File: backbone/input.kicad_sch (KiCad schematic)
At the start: 0 parts

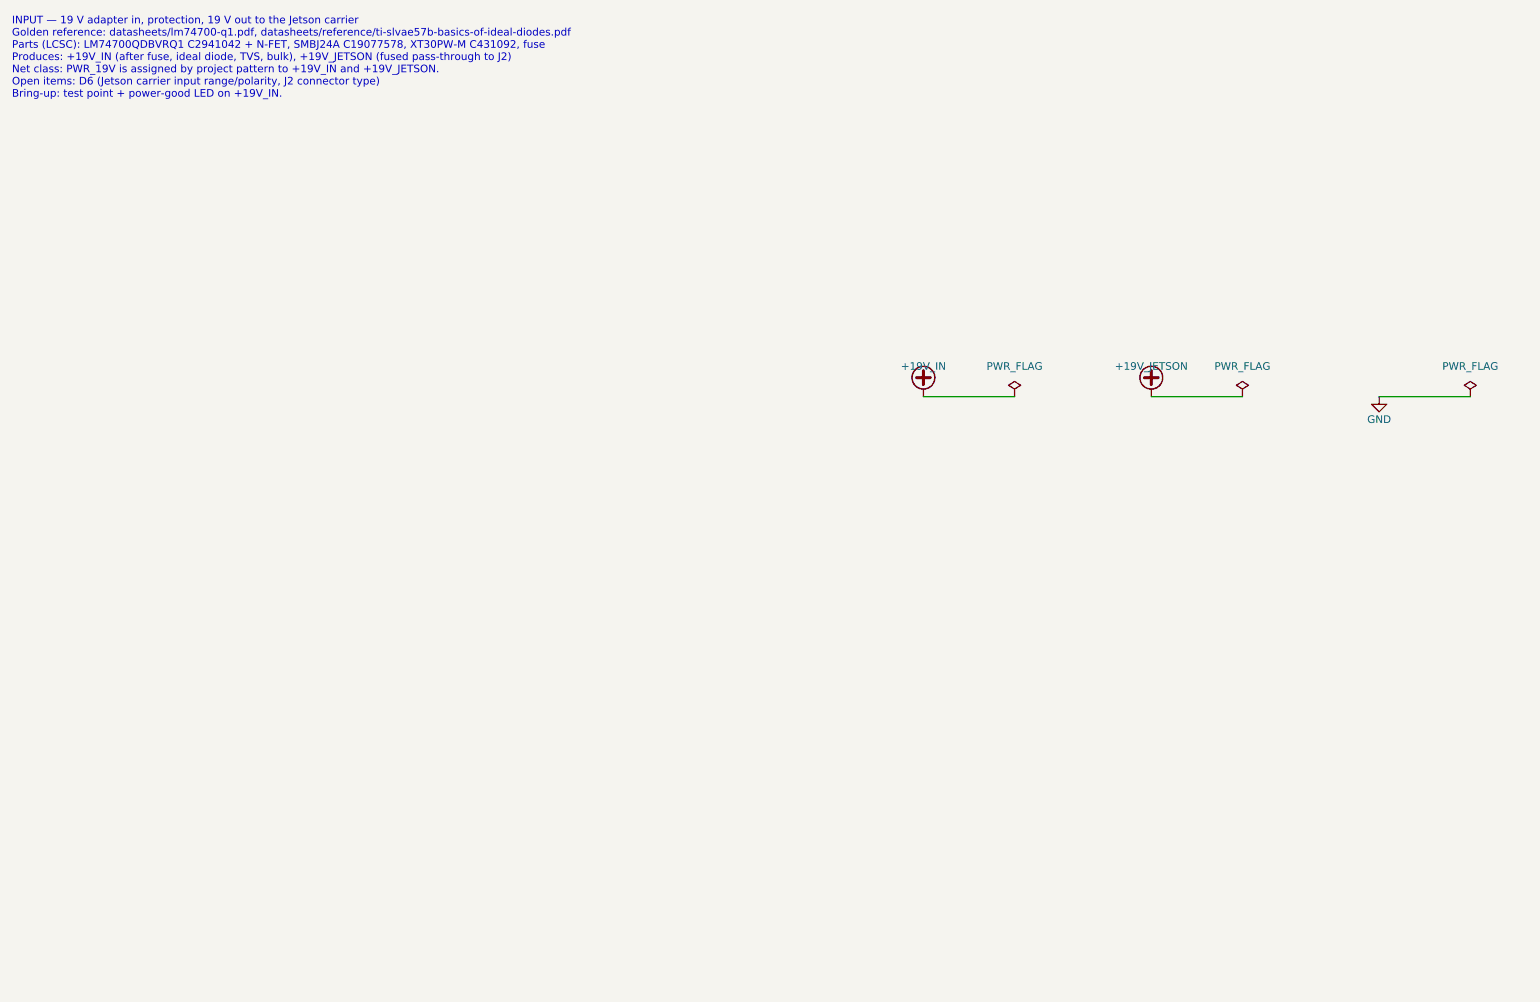
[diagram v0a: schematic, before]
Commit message: before hand editing
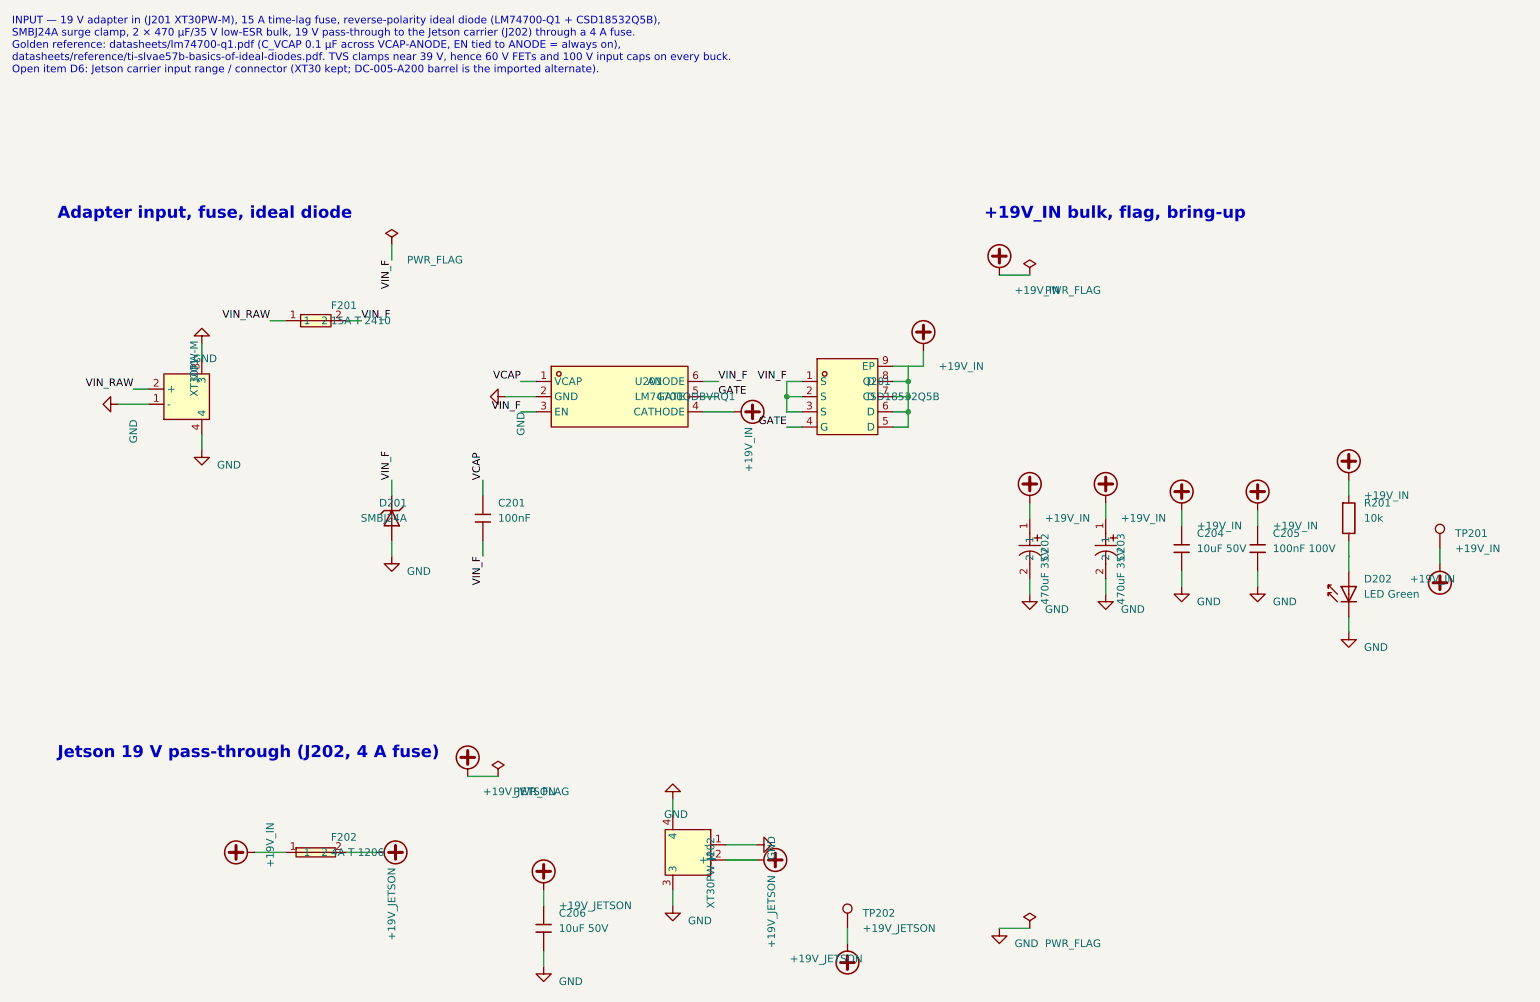
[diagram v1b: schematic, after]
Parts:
- added C201: 100nF, 0_backbone:C_0603, symbol 0_backbone:C_0603
- added C202, C203: 470uF 35V, 0_backbone:CAP-SMD_BD10.0-L10.3-W10.3-LS11.3-FD, symbol 0_backbone:RVE470UF35V167RV084
- added C204, C206: 10uF 50V, 0_backbone:C_1206, symbol 0_backbone:C_1206
- added C205: 100nF 100V, 0_backbone:C_0805, symbol 0_backbone:C_0805
- added D201: SMBJ24A, 0_backbone:D_SMB, symbol 0_backbone:TVS_SMB
- added D202: LED Green, 0_backbone:D_0805, symbol 0_backbone:LED_0805_Green
- added F201: 15A T 2410, 0_backbone:FUSE-SMD_L6.1-W2.7, symbol 0_backbone:0453015.MR
- added F202: 4A T 1206, 0_backbone:F1206, symbol 0_backbone:1206TD-4A
- added J201, J202: XT30PW-M, 0_backbone:CONN-TH_XT30PW-M, symbol 0_backbone:XT30PW-M
- added Q201: CSD18532Q5B, 0_backbone:SON-8_L5.0-W6.0-P1.27-BL-1, symbol 0_backbone:CSD18532Q5B
- added R201: 10k, 0_backbone:R_0603, symbol 0_backbone:R_0603
- added TP201: +19V_IN, 0_backbone:TestPoint_Pad_D1.5mm, symbol 0_backbone:TestPoint
- added TP202: +19V_JETSON, 0_backbone:TestPoint_Pad_D1.5mm, symbol 0_backbone:TestPoint
- added U201: LM74700QDBVRQ1, 0_backbone:SOT-23-6_L2.9-W1.6-P0.95-LS2.8-BL, symbol 0_backbone:LM74700QDBVRQ1
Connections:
- net +19V_IN: now also C202.1, C203.1, C204.1, C205.1, F202.1, Q201.5 (D), Q201.6 (D), Q201.7 (D), Q201.8 (D), Q201.9 (EP), R201.1, TP201.1, U201.4 (CATHODE)
- net +19V_JETSON: now also C206.1, F202.2, J202.2 (+), TP202.1
- net GND: now also C202.2, C203.2, C204.2, C205.2, C206.2, D201.2, D202.1, J201.1 (-), J201.3, J201.4, J202.1 (-), J202.3, J202.4, U201.2 (GND)
- new net: D202.2, R201.2
- new net GATE: Q201.4 (G), U201.5 (GATE)
- new net VCAP: C201.1, U201.1 (VCAP)
- new net VIN_F: C201.2, D201.1, F201.2, Q201.1 (S), Q201.2 (S), Q201.3 (S), U201.3 (EN), U201.6 (ANODE)
- new net VIN_RAW: F201.1, J201.2 (+)
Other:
- note added: "+19V_IN bulk, flag, bring-up"
- note added: "Adapter input, fuse, ideal diode"
- note added: "INPUT — 19 V adapter in (J201 XT30PW-M), 15 A time-lag fuse, reverse-polarity ideal diode (LM74700-Q1 + CSD18532Q5B), SMBJ24A surge clamp, 2 × 470 µF/35 V low-ESR bulk, 19 V pass-through to the Jetson carrier (J202) through a 4 A fuse. Golden reference: datasheets/lm74700-q1.pdf (C_VCAP 0.1 µF across VCAP-ANODE, EN tied to ANODE = always on), datasheets/reference/ti-slvae57b-basics-of-ideal-diode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"
- note added: "Jetson 19 V pass-through (J202, 4 A fuse)"
- note removed: "INPUT — 19 V adapter in, protection, 19 V out to the Jetson carrier Golden reference: datasheets/lm74700-q1.pdf, datasheets/reference/ti-slvae57b-basics-of-ideal-diodes.pdf Parts (LCSC): LM74700QDBVRQ1 C2941042 + N-FET, SMBJ24A C19077578, XT30PW-M C431092, fuse Produces: +19V_IN (after fuse, ideal diode, TVS, bulk), +19V_JETSON (fused pass-through to J2) Net class: PWR_19V is assigned by project 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"

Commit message: schematics
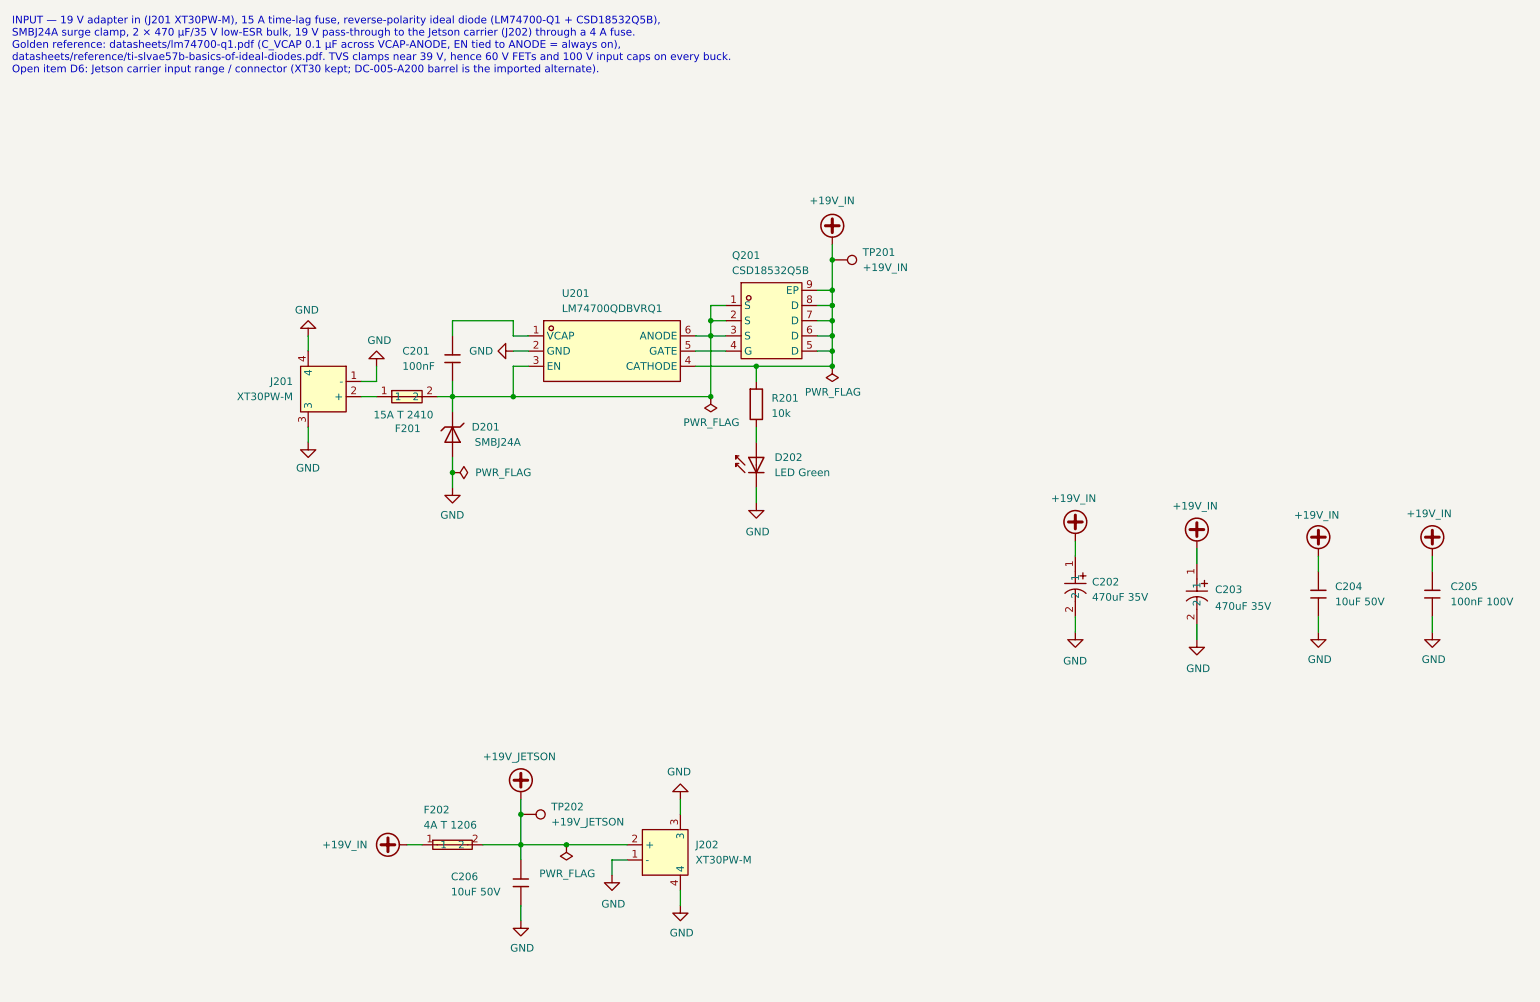
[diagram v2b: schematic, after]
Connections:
- net GATE: no longer names the net of Q201.4 (G), U201.5 (GATE)
- net VCAP: no longer names the net of C201.1, U201.1 (VCAP)
- net VIN_F: no longer names the net of C201.2, D201.1, F201.2, Q201.1 (S), Q201.2 (S), Q201.3 (S), U201.3 (EN), U201.6 (ANODE)
- net VIN_RAW: no longer names the net of F201.1, J201.2 (+)
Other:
- note removed: "+19V_IN bulk, flag, bring-up"
- note removed: "Adapter input, fuse, ideal diode"
- note removed: "Jetson 19 V pass-through (J202, 4 A fuse)"
- moved on the sheet: C201, C202, C203, C204, C205, C206, D201, D202, F201, F202, J201, J202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
